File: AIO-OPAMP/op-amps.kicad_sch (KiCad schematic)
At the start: 30 parts, among them J1 Screw_Terminal_01x02, J10 Conn_01x01_Pin, J11 Conn_01x02, J12 Conn_01x01_Pin, J13 Conn_01x01_Pin, J14 Conn_01x03, J15 Conn_01x03, J16 Conn_01x03, J17 Conn_01x03, J18 Conn_01x02, J19 Conn_01x01_Pin, J2 Conn_02x03_Odd_Even, J3 Screw_Terminal_01x03, J4 Conn_01x01_Pin, J5 Conn_01x02, J6 Conn_01x01_Pin, J7 Conn_01x01_Pin, J8 Conn_01x01_Pin, J9 Conn_01x02, U1 TL084

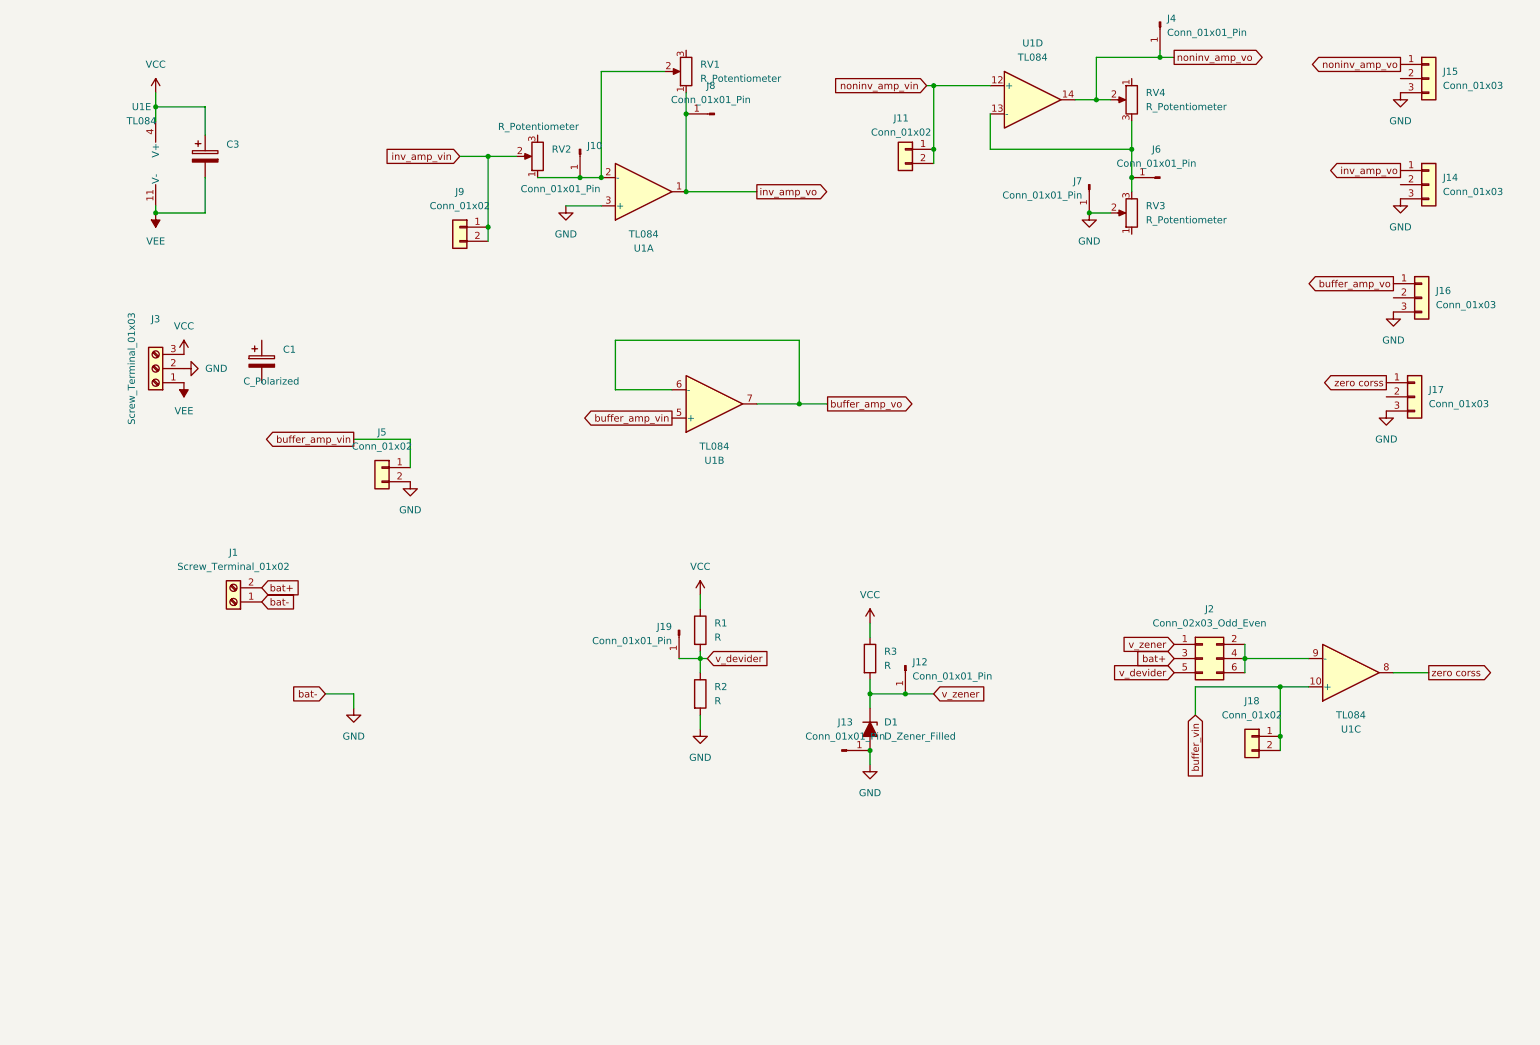
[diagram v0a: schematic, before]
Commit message: s
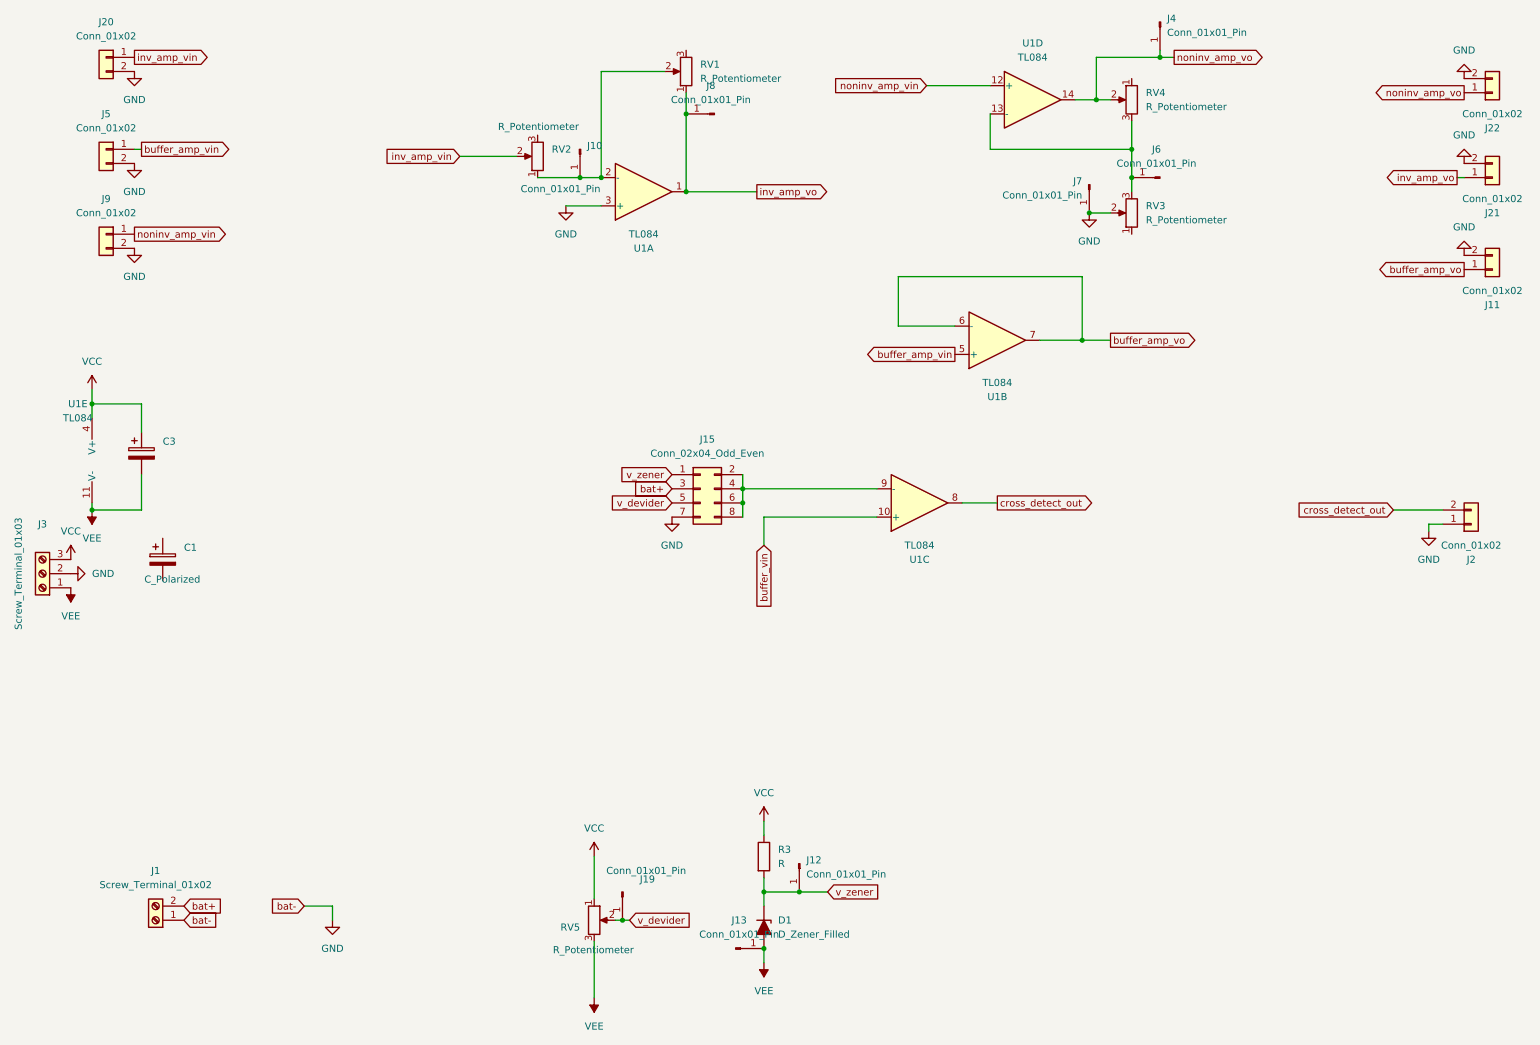
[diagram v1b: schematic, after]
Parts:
- removed J14, J15, J16, J17: Conn_01x03, Connector_PinHeader_2.54mm:PinHeader_1x03_P2.54mm_Vertical, symbol Connector_Generic:Conn_01x03
- removed J18: Conn_01x02, Connector_PinHeader_2.54mm:PinHeader_1x02_P2.54mm_Vertical, symbol Connector_Generic:Conn_01x02
- removed J2: Conn_02x03_Odd_Even, Connector_PinHeader_2.54mm:PinHeader_2x03_P2.54mm_Vertical, symbol Connector_Generic:Conn_02x03_Odd_Even
- removed R1, R2: R, Resistor_THT:R_Axial_DIN0207_L6.3mm_D2.5mm_P7.62mm_Horizontal, symbol Device:R
- added J15: Conn_02x04_Odd_Even, symbol Connector_Generic:Conn_02x04_Odd_Even
- added J2, J20, J21, J22: Conn_01x02, Connector_PinHeader_2.54mm:PinHeader_1x02_P2.54mm_Vertical, symbol Connector_Generic:Conn_01x02
- added RV5: R_Potentiometer, Potentiometer_THT:Potentiometer_Bourns_3296W_Vertical, symbol Device:R_Potentiometer
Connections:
- net GND: now also J11.2 (Pin_2), J9.2 (Pin_2), J15.7 (Pin_7), J2.1 (Pin_1), J20.2 (Pin_2), J21.2 (Pin_2), J22.2 (Pin_2); no longer D1.2 (A), J13.1 (Pin_1)
- net VCC: now also RV5.1
- net VEE: now also D1.2 (A), J13.1 (Pin_1), RV5.3
- net bat+: now also J15.3 (Pin_3)
- net buffer_amp_vo: now also J11.1 (Pin_1)
- net inv_amp_vin: now also J20.1 (Pin_1); no longer J9.1 (Pin_1), J9.2 (Pin_2)
- net inv_amp_vo: now also J21.1 (Pin_1)
- net noninv_amp_vin: now also J9.1 (Pin_1); no longer J11.1 (Pin_1), J11.2 (Pin_2)
- net noninv_amp_vo: now also J22.1 (Pin_1)
- net v_devider: now also J15.5 (Pin_5), RV5.2
- net v_zener: now also J15.1 (Pin_1)
- net at U1.9 (-): now also J15.2 (Pin_2), J15.4 (Pin_4), J15.6 (Pin_6), J15.8 (Pin_8)
- net zero corss renamed cross_detect_out
- net cross_detect_out: now also J2.2 (Pin_2)
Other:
- moved on the sheet: C1, C3, D1, J1, J12, J13, J19, J3, J5, R3, U1B, U1C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
